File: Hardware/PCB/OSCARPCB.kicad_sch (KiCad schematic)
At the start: 7 parts, among them J1 PINHD_1x8_Male, J2 PINHD_1x8_Male, J4 Servo OUT, J5 Power Input, J6 PINHD_1x2_Female, U2 ESP32-DevKitC

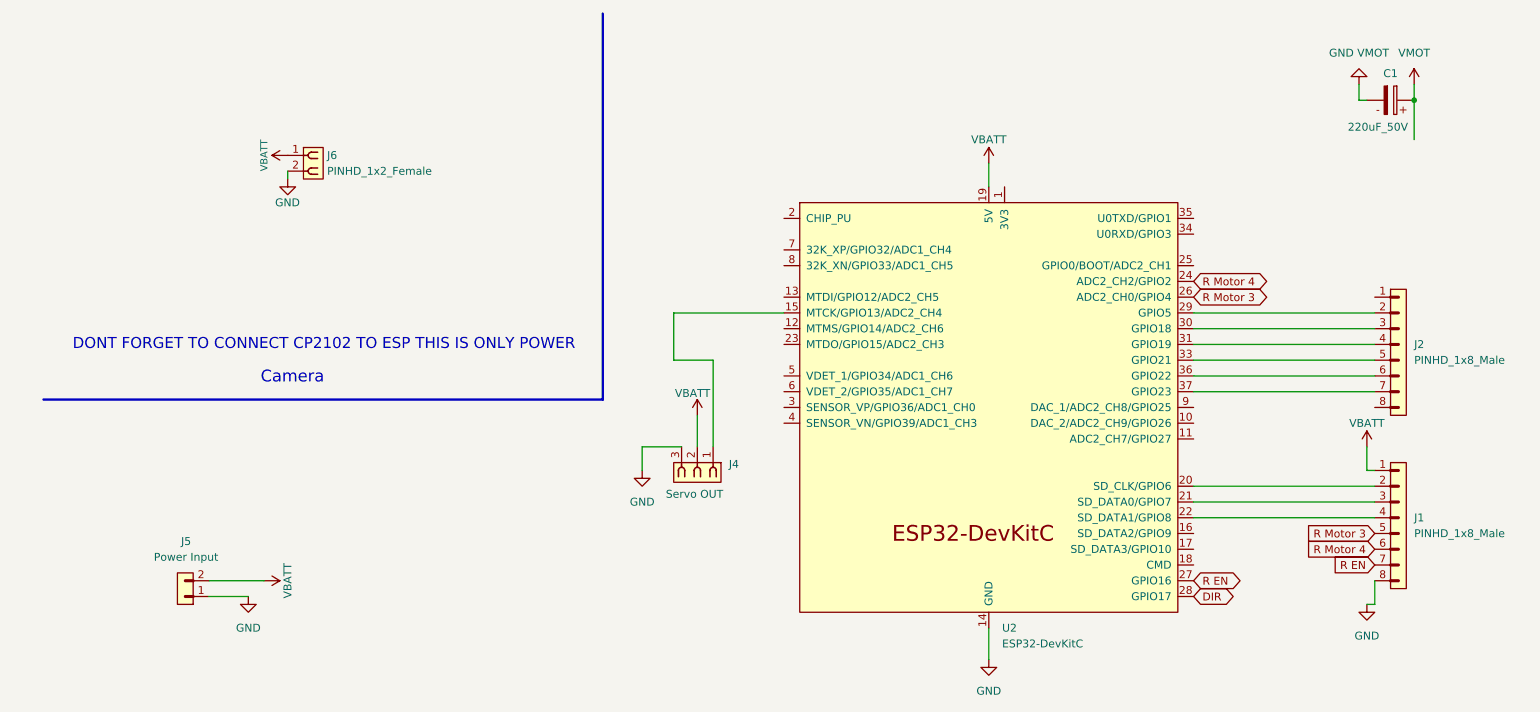
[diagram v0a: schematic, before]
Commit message: PCB Done?
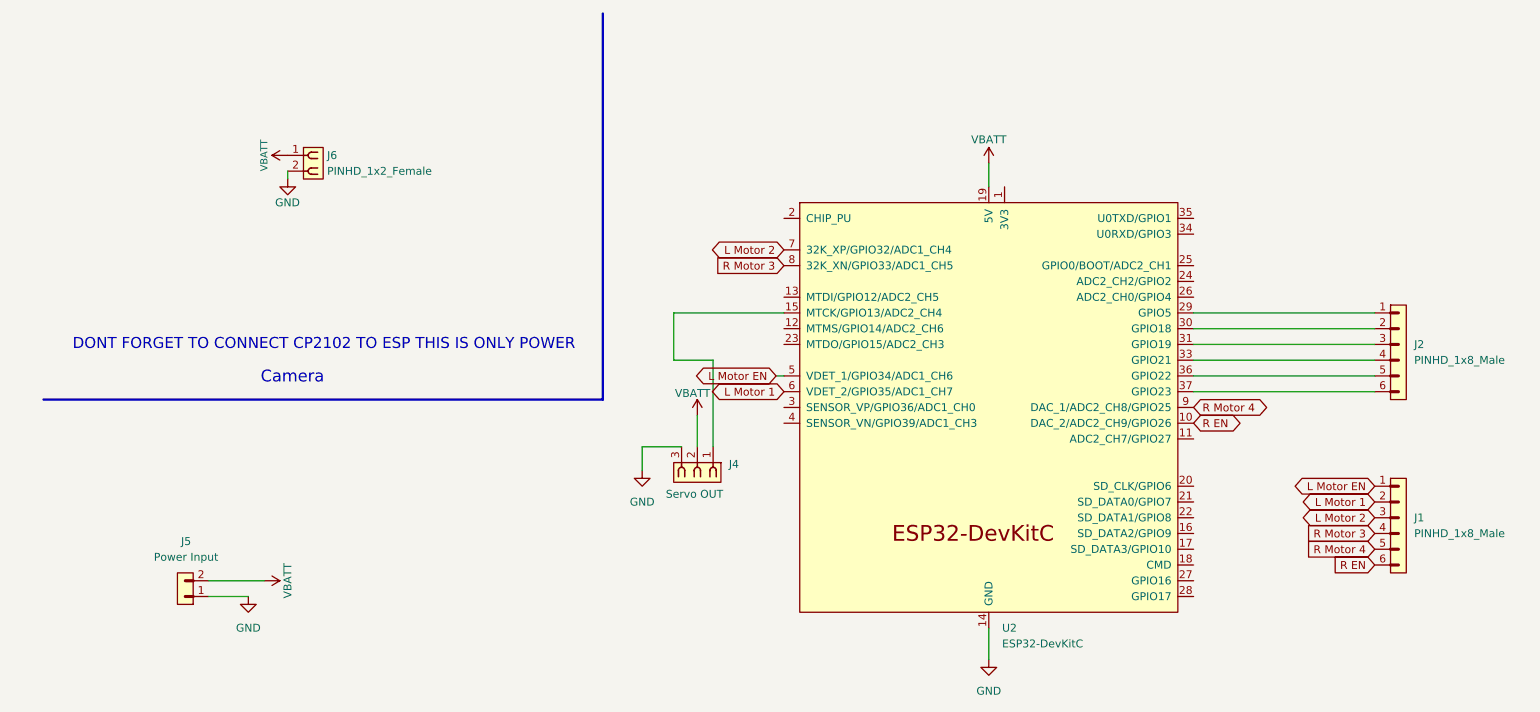
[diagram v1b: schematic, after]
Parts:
- removed C1: 220uF_50V, Capacitor_THT:CP_Radial_D10.0mm_P5.00mm, symbol PCM_SL_Capacitors:220uF_50V
- J1, J2: footprint Connector_PinHeader_2.54mm:PinHeader_1x08_P2.54mm_Vertical -> Connector_PinHeader_2.54mm:PinHeader_1x06_P2.54mm_Vertical; symbol PCM_SL_Pin_Headers:PINHD_1x8_Male -> PCM_SL_Pin_Headers:PINHD_1x6_Male
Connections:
- net GND: no longer J1.8
- net R EN: now also J1.6, U2.10 (DAC_2/ADC2_CH9/GPIO26); no longer J1.7, U2.27 (GPIO16)
- net R Motor 3: now also J1.4, U2.8 (32K_XN/GPIO33/ADC1_CH5); no longer J1.5, U2.26 (ADC2_CH0/GPIO4)
- net R Motor 4: now also J1.5, U2.9 (DAC_1/ADC2_CH8/GPIO25); no longer J1.6, U2.24 (ADC2_CH2/GPIO2)
- net VBATT: no longer J1.1
- net at J2.1: now also U2.29 (GPIO5)
- net at J2.2: now also U2.30 (GPIO18); no longer U2.29 (GPIO5)
- net at J2.3: now also U2.31 (GPIO19); no longer U2.30 (GPIO18)
- net at J2.4: now also U2.33 (GPIO21); no longer U2.31 (GPIO19)
- net at J2.5: now also U2.36 (GPIO22); no longer U2.33 (GPIO21)
- net at J2.6: now also U2.37 (GPIO23); no longer U2.36 (GPIO22)
- net at U2.20 (SD_CLK/GPIO6): no longer J1.2
- net at U2.21 (SD_DATA0/GPIO7): no longer J1.3
- net at U2.22 (SD_DATA1/GPIO8): no longer J1.4
- net L Motor EN: now reaches U2.5 (VDET_1/GPIO34/ADC1_CH6)
- net L Motor EN: now also J1.1
- net L Motor 1: now reaches U2.6 (VDET_2/GPIO35/ADC1_CH7)
- net L Motor 1: now also J1.2
- net L Motor 2: now reaches U2.7 (32K_XP/GPIO32/ADC1_CH4)
- net L Motor 2: now also J1.3
- net DIR: no longer names the net of U2.28 (GPIO17)
